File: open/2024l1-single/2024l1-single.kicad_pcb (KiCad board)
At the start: 2 copper layers, 176 x 169.5 mm, 96 parts, among them IC1 LM2587S-ADJ, J1 Conn_01x03, J2 Conn_01x03, J3 Conn_01x02, J4 Conn_01x02, J5 XT30, J6 Conn_01x04, Q1 STP75NF75, Q2 STP75NF75, U1 Seeed Studio XIAO SAMD21, U2 CD74HC4067SM

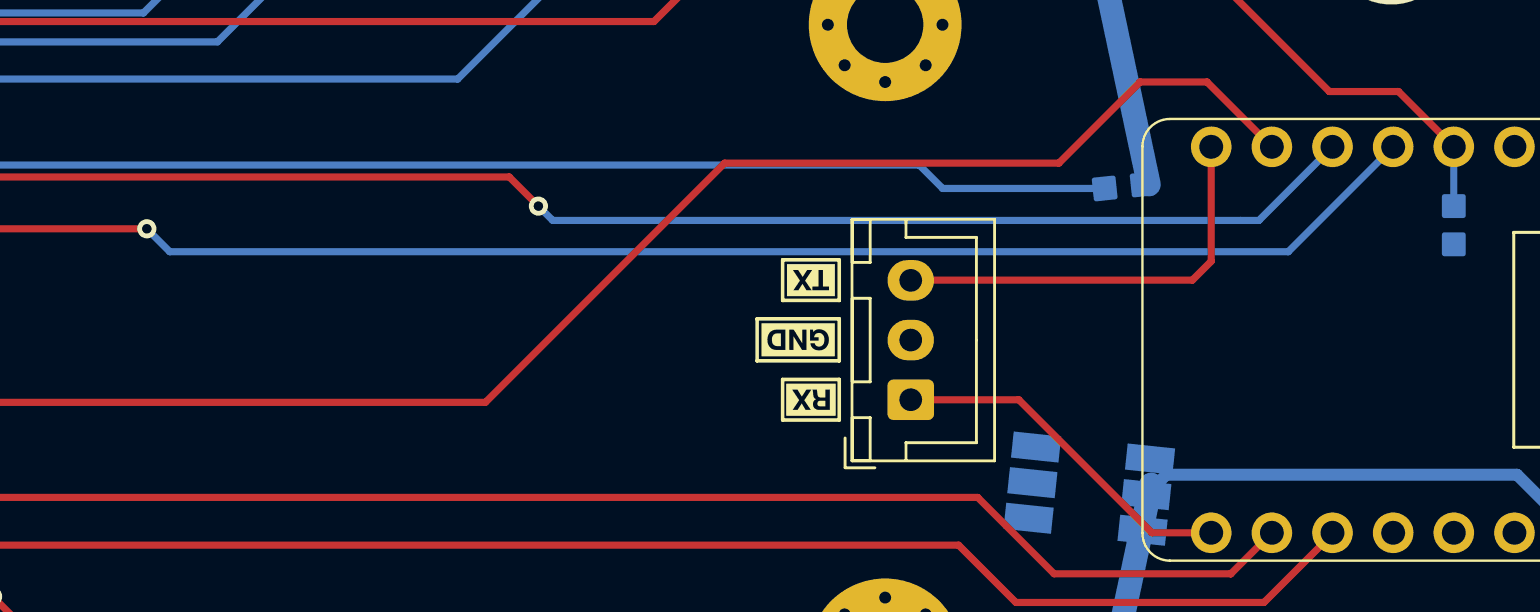
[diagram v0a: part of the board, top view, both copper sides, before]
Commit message: L1 Minor adjust and l2 still need to add stitching vias
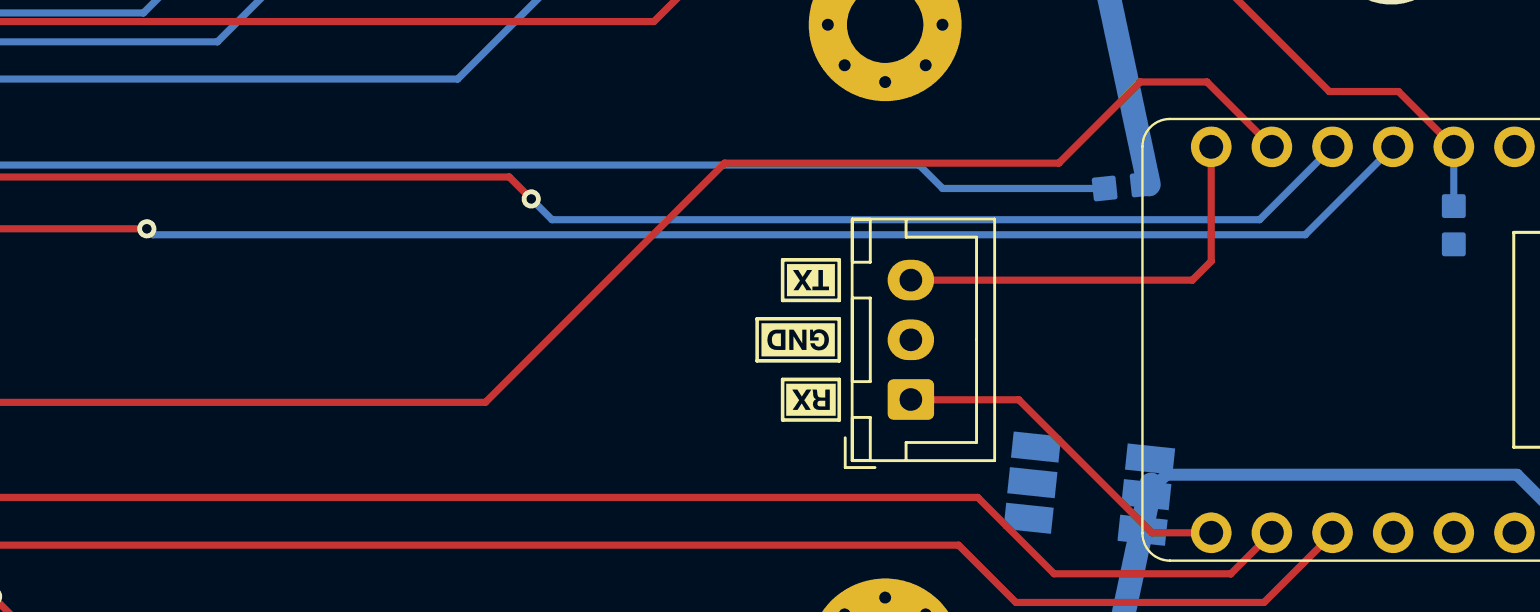
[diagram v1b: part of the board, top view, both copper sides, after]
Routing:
- net /S3: track 67.4 -> 66.8 mm
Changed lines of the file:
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@@
   )
   (footprint "Connector_JST:JST_XH_B3B-XH-A_1x03_P2.50mm_Vertical" (layer "F.Cu")
-    (at 159.495 114.76 90)
+    (at 159.5 114.75 90)
     (descr "JST XH series connector, B3B-XH-A (http://www.jst-mfg.com/product/pdf/eng/eXH.pdf), generated with kicad-footprint-generator")
     (tags "connector JST XH vertical")
@@
   (segment (start 114.495 107.6) (end 114.485 107.61) (width 0.3) (layer "F.Cu") (net 44))
   (via (at 127.5 107.6) (size 0.8) (drill 0.4) (layers "F.Cu" "B.Cu") (net 44))
-  (segment (start 128.46 108.56) (end 127.5 107.6) (width 0.3) (layer "B.Cu") (net 44))
-  (segment (start 179.7 104.1675) (end 175.3075 108.56) (width 0.3) (layer "B.Cu") (net 44))
-  (segment (start 175.3075 108.56) (end 128.46 108.56) (width 0.3) (layer "B.Cu") (net 44))
-  (segment (start 113.215 106.405) (end 113.215 107.61) (width 0.3) (layer "F.Cu") (net 45))
-  (segment (start 114.19 105.43) (end 113.215 106.405) (width 0.3) (layer "F.Cu") (net 45))
-  (segment (start 143.9 106.65) (end 142.68 105.43) (width 0.3) (layer "F.Cu") (net 45))
+  (segment (start 127.75 107.85) (end 127.5 107.6) (width 0.3) (layer "B.Cu") (net 44))
+  (segment (start 176.0175 107.85) (end 127.75 107.85) (width 0.3) (layer "B.Cu") (net 44))
+  (segment (start 179.7 104.1675) (end 176.0175 107.85) (width 0.3) (layer "B.Cu") (net 44))
   (segment (start 142.68 105.43) (end 114.19 105.43) (width 0.3) (layer "F.Cu") (net 45))
-  (via (at 143.9 106.65) (size 0.8) (drill 0.4) (layers "F.Cu" "B.Cu") (net 45))
-  (segment (start 174.0775 107.25) (end 173.3 107.25) (width 0.3) (layer "B.Cu") (net 45))
-  (segment (start 143.9 106.65) (end 144.5 107.25) (width 0.3) (layer "B.Cu") (net 45))
-  (segment (start 144.5 107.25) (end 173.3 107.25) (width 0.3) (layer "B.Cu") (net 45))
-  (segment (start 177.16 104.1675) (end 174.0775 107.25) (width 0.3) (layer "B.Cu") (net 45))
+  (segment (start 143.6 106.35) (end 142.68 105.43) (width 0.3) (layer "F.Cu") (net 45))
+  (segment (start 114.19 105.43) (end 113.215 106.405) (width 0.3) (layer "F.Cu") (net 45))
+  (segment (start 113.215 106.405) (end 113.215 107.61) (width 0.3) (layer "F.Cu") (net 45))
+  (via (at 143.6 106.35) (size 0.8) (drill 0.4) (layers "F.Cu" "B.Cu") (net 45))
+  (segment (start 174.1075 107.22) (end 177.16 104.1675) (width 0.3) (layer "B.Cu") (net 45))
+  (segment (start 143.6 106.35) (end 144.47 107.22) (width 0.3) (layer "B.Cu") (net 45))
+  (segment (start 144.47 107.22) (end 174.1075 107.22) (width 0.3) (layer "B.Cu") (net 45))
   (segment (start 169.5925 120.3325) (end 172.08 120.3325) (width 0.3) (layer "F.Cu") (net 46))
   (segment (start 159.495 114.76) (end 164.02 114.76) (width 0.3) (layer "F.Cu") (net 46))
